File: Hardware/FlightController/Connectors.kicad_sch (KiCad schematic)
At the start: 14 parts, among them J10 Conn_01x03, J11 Conn_01x04, J13 Conn_01x02, J2 USB_B_Mini, J3 Conn_02x03_Odd_Even, J4 Conn_01x04, J5 Conn_01x03, J6 Conn_01x03, J7 Conn_01x03, J8 Conn_01x03, J9 Conn_01x03

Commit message: Update footprints to be digikey compliant
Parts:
- J2: footprint Connector_USB:USB_Mini-B_Lumberg_2486_01_Horizontal -> digikey-footprints:USB_Mini_B_Female_UX60-MB-5ST
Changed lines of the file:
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@@
     (property "Reference" "J2" (id 0) (at 101.6 134.62 0))
     (property "Value" "USB_B_Mini" (id 1) (at 101.6 137.16 0))
-    (property "Footprint" "Connector_USB:USB_Mini-B_Lumberg_2486_01_Horizontal" (id 2) (at 105.41 148.59 0)
+    (property "Footprint" "digikey-footprints:USB_Mini_B_Female_UX60-MB-5ST" (id 2) (at 105.41 148.59 0)
       (effects (font (size 1.27 1.27)) hide)
     )

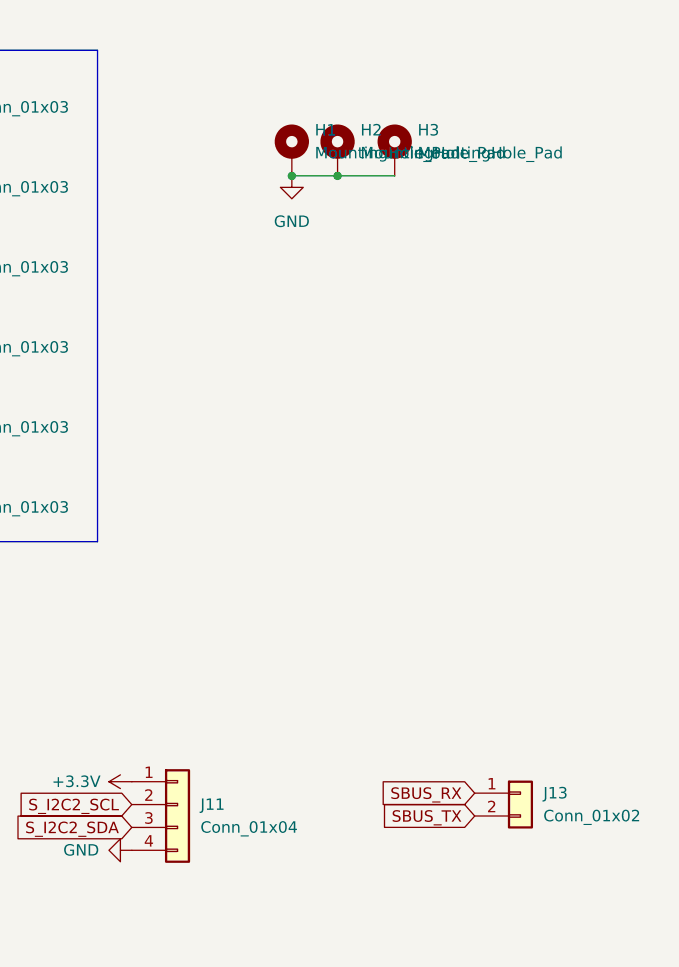
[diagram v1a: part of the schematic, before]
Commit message: Update footprints, routing and LCSC numbers
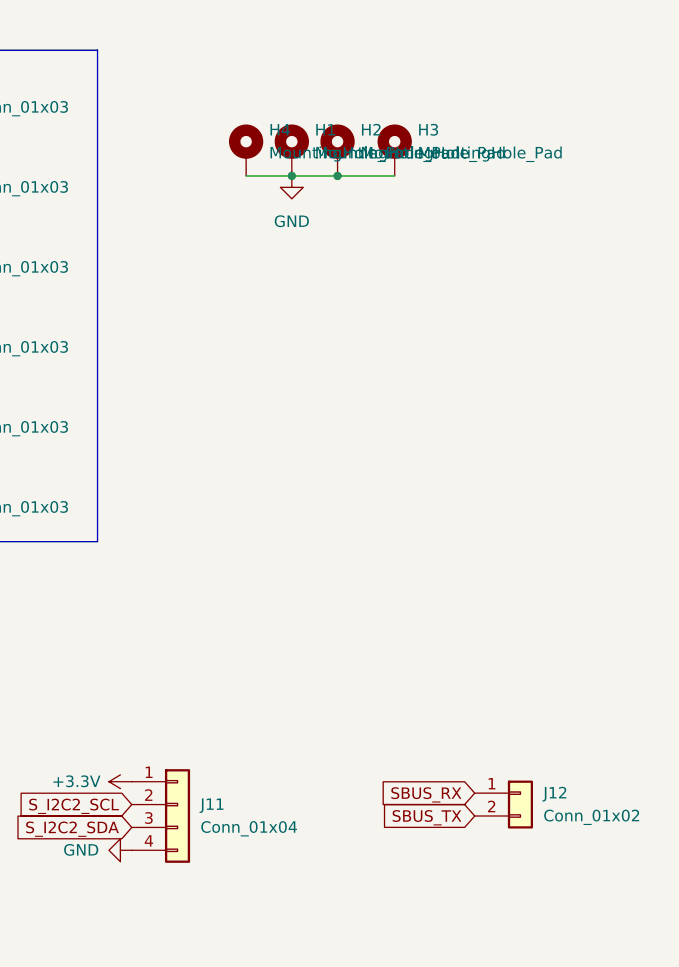
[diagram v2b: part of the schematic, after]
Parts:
- added H4: MountingHole_Pad, MountingHole:MountingHole_2.5mm_Pad, symbol Mechanical:MountingHole_Pad
- renumbered J13 to J12
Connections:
- net GND: now also H4.1
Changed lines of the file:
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@@
+    (stroke (width 0) (type default) (color 0 0 0 0))
+  )
+  (wire (pts (xy 166.37 39.37) (xy 171.45 39.37))
     (stroke (width 0) (type default) (color 0 0 0 0))
   )
@@
   (symbol (lib_id "power:GND") (at 128.27 50.8 270) (unit 1)
     (in_bom yes) (on_board yes) (fields_autoplaced)
-    (property "Reference" "#PWR0128" (id 0) (at 121.92 50.8 0)
+    (property "Reference" "#PWR038" (id 0) (at 121.92 50.8 0)
       (effects (font (size 1.27 1.27)) hide)
     )
@@
   (symbol (lib_id "power:+5V") (at 128.27 39.37 90) (unit 1)
     (in_bom yes) (on_board yes) (fields_autoplaced)
-    (property "Reference" "#PWR0125" (id 0) (at 132.08 39.37 0)
+    (property "Reference" "#PWR035" (id 0) (at 132.08 39.37 0)
       (effects (font (size 1.27 1.27)) hide)
     )
@@
   (symbol (lib_id "power:GND") (at 105.41 109.22 270) (unit 1)
     (in_bom yes) (on_board yes)
-    (property "Reference" "#PWR0117" (id 0) (at 99.06 109.22 0)
+    (property "Reference" "#PWR030" (id 0) (at 99.06 109.22 0)
       (effects (font (size 1.27 1.27)) hide)
     )
@@
   (symbol (lib_id "power:GND") (at 101.6 157.48 0) (unit 1)
     (in_bom yes) (on_board yes) (fields_autoplaced)
-    (property "Reference" "#PWR0116" (id 0) (at 101.6 163.83 0)
+    (property "Reference" "#PWR028" (id 0) (at 101.6 163.83 0)
       (effects (font (size 1.27 1.27)) hide)
     )
@@
   (symbol (lib_id "power:+5V") (at 128.27 66.04 90) (unit 1)
     (in_bom yes) (on_board yes) (fields_autoplaced)
-    (property "Reference" "#PWR0109" (id 0) (at 132.08 66.04 0)
+    (property "Reference" "#PWR041" (id 0) (at 132.08 66.04 0)
       (effects (font (size 1.27 1.27)) hide)
     )
@@
   (symbol (lib_id "power:GND") (at 110.49 129.54 270) (unit 1)
     (in_bom yes) (on_board yes)
-    (property "Reference" "#PWR0120" (id 0) (at 104.14 129.54 0)
+    (property "Reference" "#PWR032" (id 0) (at 104.14 129.54 0)
       (effects (font (size 1.27 1.27)) hide)
     )
@@
   (symbol (lib_id "power:+3.3V") (at 153.67 106.68 90) (mirror x) (unit 1)
     (in_bom yes) (on_board yes)
-    (property "Reference" "#PWR0105" (id 0) (at 157.48 106.68 0)
+    (property "Reference" "#PWR045" (id 0) (at 157.48 106.68 0)
       (effects (font (size 1.27 1.27)) hide)
     )
@@
   (symbol (lib_id "power:GND") (at 128.27 77.47 270) (unit 1)
     (in_bom yes) (on_board yes) (fields_autoplaced)
-    (property "Reference" "#PWR0122" (id 0) (at 121.92 77.47 0)
+    (property "Reference" "#PWR044" (id 0) (at 121.92 77.47 0)
       (effects (font (size 1.27 1.27)) hide)
     )
@@
   (symbol (lib_id "power:+3.3V") (at 110.49 121.92 90) (mirror x) (unit 1)
     (in_bom yes) (on_board yes)
-    (property "Reference" "#PWR0119" (id 0) (at 114.3 121.92 0)
+    (property "Reference" "#PWR031" (id 0) (at 114.3 121.92 0)
       (effects (font (size 1.27 1.27)) hide)
     )
@@
   (symbol (lib_id "power:GND") (at 128.27 41.91 270) (unit 1)
     (in_bom yes) (on_board yes) (fields_autoplaced)
-    (property "Reference" "#PWR0123" (id 0) (at 121.92 41.91 0)
+    (property "Reference" "#PWR036" (id 0) (at 121.92 41.91 0)
       (effects (font (size 1.27 1.27)) hide)
     )
@@
   (symbol (lib_id "power:+5V") (at 128.27 57.15 90) (unit 1)
     (in_bom yes) (on_board yes) (fields_autoplaced)
-    (property "Reference" "#PWR0106" (id 0) (at 132.08 57.15 0)
+    (property "Reference" "#PWR039" (id 0) (at 132.08 57.15 0)
       (effects (font (size 1.27 1.27)) hide)
     )
@@
     (pin "1")
   )
+  (symbol (lib_id "Mechanical:MountingHole_Pad") (at 166.37 36.83 0) (unit 1)
+    (in_bom yes) (on_board yes) (fields_autoplaced)
+    (property "Reference" "H4" (id 0) (at 168.91 34.2899 0)
+      (effects (font (size 1.27 1.27)) (justify left))
+    )
+    (property "Value" "MountingHole_Pad" (id 1) (at 168.91 36.8299 0)
+      (effects (font (size 1.27 1.27)) (justify left))
+    )
+    (property "Footprint" "MountingHole:MountingHole_2.5mm_Pad" (id 2) (at 166.37 36.83 0)
+      (effects (font (size 1.27 1.27)) hide)
+    )
+    (property "Datasheet" "~" (id 3) (at 166.37 36.83 0)
+      (effects (font (size 1.27 1.27)) hide)
+    )
+    (pin "1")
+  )
   (symbol (lib_id "Connector_Generic:Conn_01x03") (at 133.35 48.26 0) (unit 1)
     (in_bom yes) (on_board yes) (fields_autoplaced)
@@
   (symbol (lib_id "power:GND") (at 128.27 59.69 270) (unit 1)
     (in_bom yes) (on_board yes) (fields_autoplaced)
-    (property "Reference" "#PWR0108" (id 0) (at 121.92 59.69 0)
+    (property "Reference" "#PWR040" (id 0) (at 121.92 59.69 0)
       (effects (font (size 1.27 1.27)) hide)
     )
@@
   (symbol (lib_id "power:+5V") (at 128.27 48.26 90) (unit 1)
     (in_bom yes) (on_board yes) (fields_autoplaced)
-    (property "Reference" "#PWR0127" (id 0) (at 132.08 48.26 0)
+    (property "Reference" "#PWR037" (id 0) (at 132.08 48.26 0)
       (effects (font (size 1.27 1.27)) hide)
     )
@@
   (symbol (lib_id "power:GND") (at 153.67 114.3 270) (unit 1)
     (in_bom yes) (on_board yes)
-    (property "Reference" "#PWR0104" (id 0) (at 147.32 114.3 0)
+    (property "Reference" "#PWR046" (id 0) (at 147.32 114.3 0)
       (effects (font (size 1.27 1.27)) hide)
     )
@@
   (symbol (lib_id "power:GND") (at 128.27 33.02 270) (unit 1)
     (in_bom yes) (on_board yes) (fields_autoplaced)
-    (property "Reference" "#PWR0126" (id 0) (at 121.92 33.02 0)
+    (property "Reference" "#PWR034" (id 0) (at 121.92 33.02 0)
       (effects (font (size 1.27 1.27)) hide)
     )
@@
   (symbol (lib_id "power:+5V") (at 128.27 30.48 90) (unit 1)
     (in_bom yes) (on_board yes) (fields_autoplaced)
-    (property "Reference" "#PWR0124" (id 0) (at 132.08 30.48 0)
+    (property "Reference" "#PWR033" (id 0) (at 132.08 30.48 0)
       (effects (font (size 1.27 1.27)) hide)
     )
@@
   (symbol (lib_id "power:+3.3V") (at 105.41 106.68 90) (mirror x) (unit 1)
     (in_bom yes) (on_board yes)
-    (property "Reference" "#PWR0118" (id 0) (at 109.22 106.68 0)
+    (property "Reference" "#PWR029" (id 0) (at 109.22 106.68 0)
       (effects (font (size 1.27 1.27)) hide)
     )
@@
   (symbol (lib_id "power:GND") (at 128.27 68.58 270) (unit 1)
     (in_bom yes) (on_board yes) (fields_autoplaced)
-    (property "Reference" "#PWR0107" (id 0) (at 121.92 68.58 0)
+    (property "Reference" "#PWR042" (id 0) (at 121.92 68.58 0)
       (effects (font (size 1.27 1.27)) hide)
     )
@@
   (symbol (lib_id "Connector_Generic:Conn_01x02") (at 196.85 107.95 0) (unit 1)
     (in_bom yes) (on_board yes) (fields_autoplaced)
-    (property "Reference" "J13" (id 0) (at 199.39 107.9499 0)
+    (property "Reference" "J12" (id 0) (at 199.39 107.9499 0)
       (effects (font (size 1.27 1.27)) (justify left))
     )
@@
   (symbol (lib_id "power:GND") (at 171.45 39.37 0) (unit 1)
     (in_bom yes) (on_board yes) (fields_autoplaced)
-    (property "Reference" "#PWR010" (id 0) (at 171.45 45.72 0)
+    (property "Reference" "#PWR047" (id 0) (at 171.45 45.72 0)
       (effects (font (size 1.27 1.27)) hide)
     )
@@
   (symbol (lib_id "power:+5V") (at 128.27 74.93 90) (unit 1)
     (in_bom yes) (on_board yes) (fields_autoplaced)
-    (property "Reference" "#PWR0121" (id 0) (at 132.08 74.93 0)
-      (effects (font (size 1.27 1.27)) hide)
-    )
+    (property "Reference" "#PWR043" (id 0) (at 132.08 74.93 0)
+      (effects (font (size 1.27 1.27)) hide)
+    )

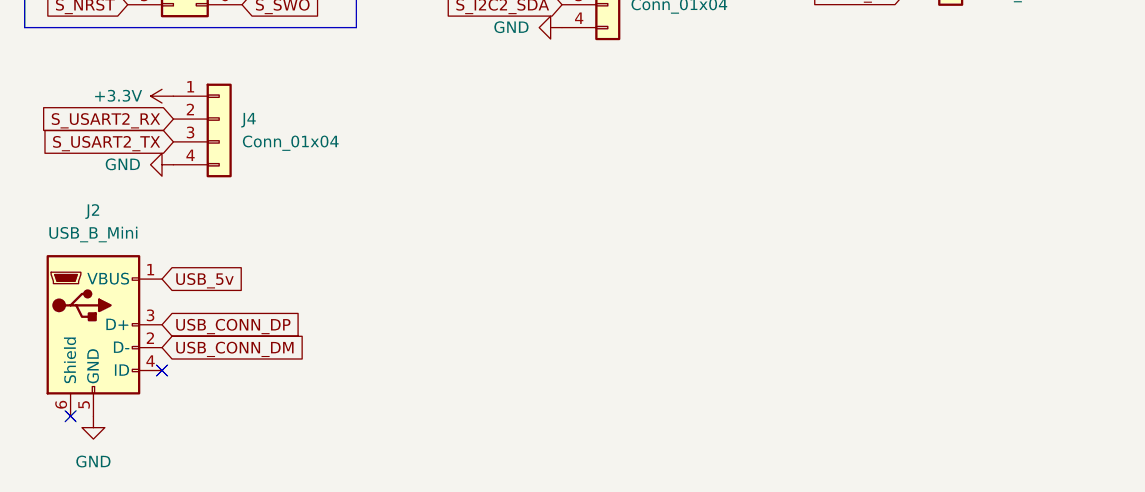
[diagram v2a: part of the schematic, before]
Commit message: Finalize design and routing for v1.0 fab
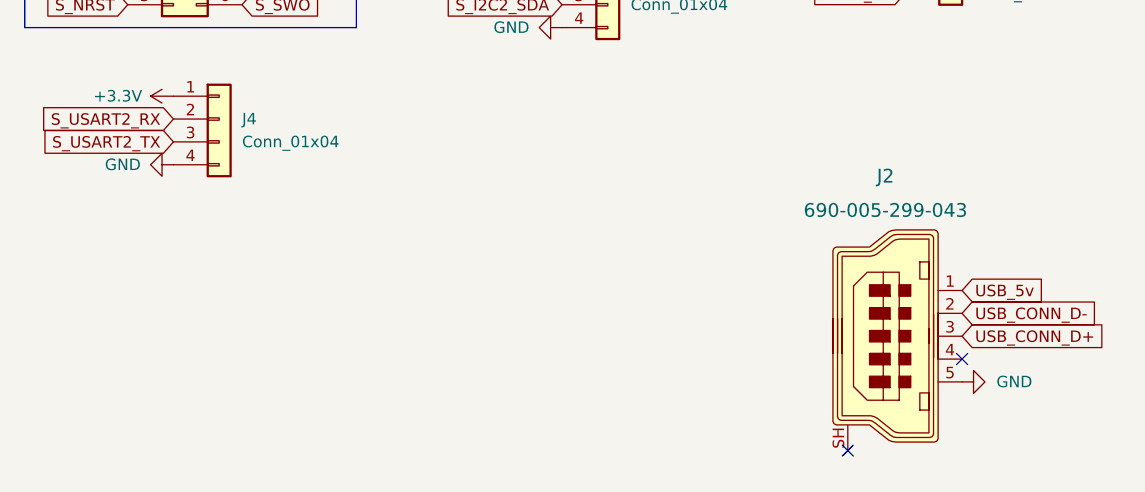
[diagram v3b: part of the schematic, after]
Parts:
- removed J2: USB_B_Mini, digikey-footprints:USB_Mini_B_Female_UX60-MB-5ST, symbol Connector:USB_B_Mini
- added J2: 690-005-299-043, digikey-footprints:USB_Mini_B_Female_690-005-299-043, symbol dk_USB-DVI-HDMI-Connectors:690-005-299-043
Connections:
- net GND: now also J2.5
- net USB_5v: now also J2.1
- new net USB_CONN_D+: J2.3
- new net USB_CONN_D-: J2.2
